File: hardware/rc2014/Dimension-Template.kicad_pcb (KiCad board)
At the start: 2 copper layers, 99.1 x 49.9 mm, 3 parts

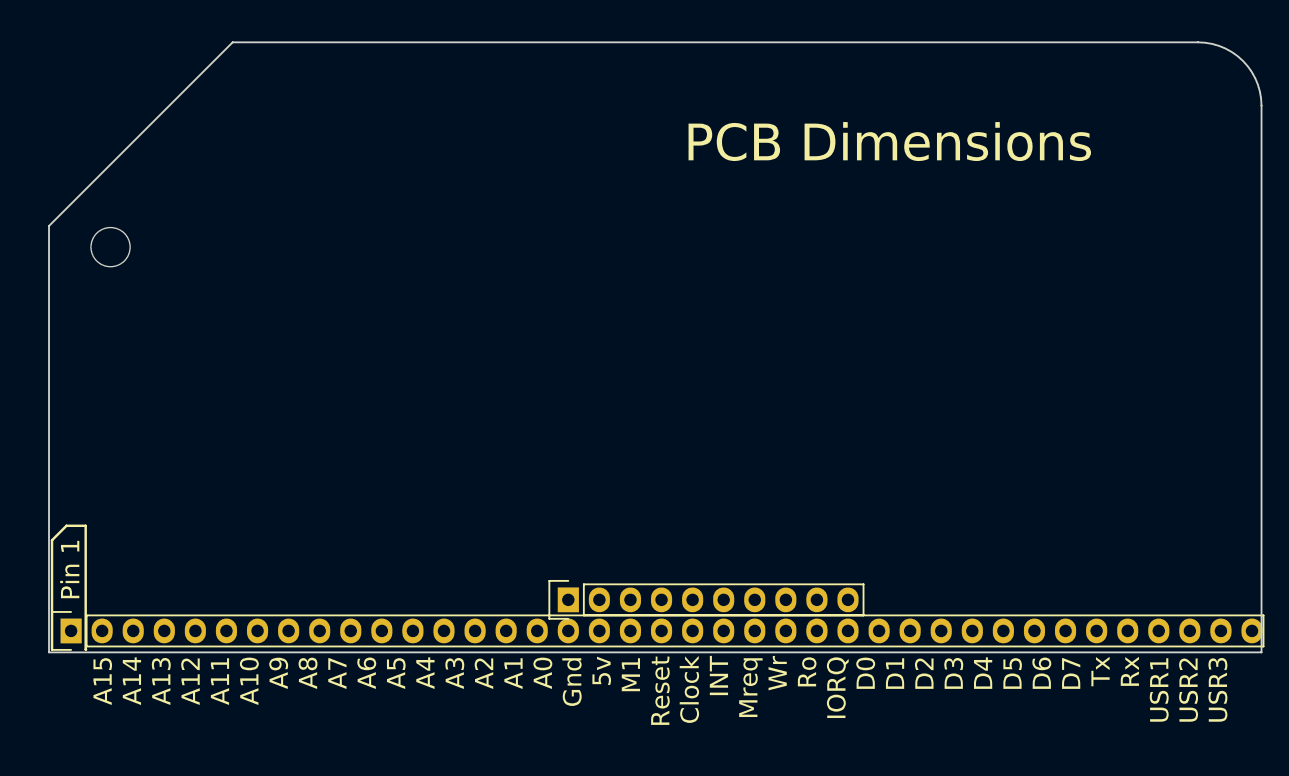
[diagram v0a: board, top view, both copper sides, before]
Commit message: more more cleaning
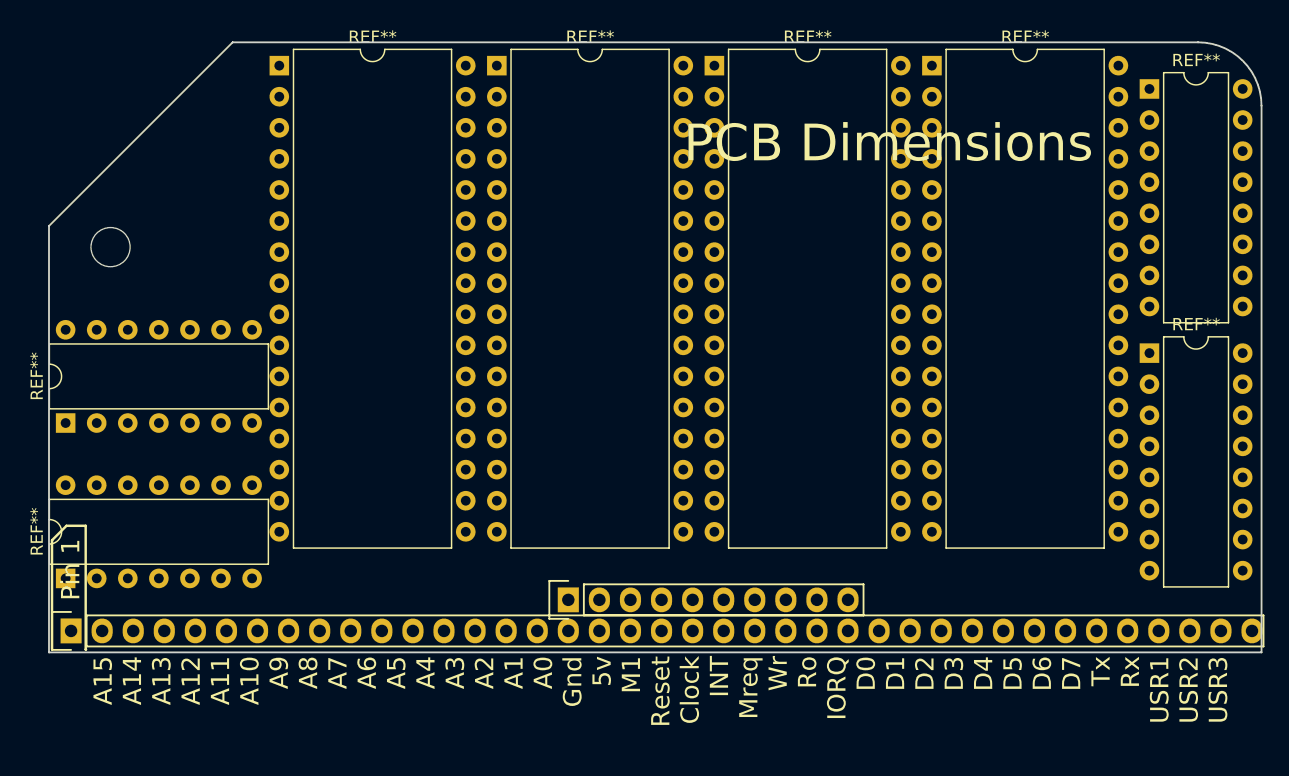
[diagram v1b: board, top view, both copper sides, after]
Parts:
- added REF**: DIP-14_W7.62mm, Package_DIP:DIP-14_W7.62mm, F.Cu at (155.3, 134.6)
- added REF**: DIP-14_W7.62mm, Package_DIP:DIP-14_W7.62mm, F.Cu at (155.3, 147.3)
- added REF**: DIP-16_W7.62mm, Package_DIP:DIP-16_W7.62mm, F.Cu at (243.8, 128.9)
- added REF**: DIP-16_W7.62mm, Package_DIP:DIP-16_W7.62mm, F.Cu at (243.8, 107.3)
- added REF**: DIP-32_W15.24mm, Package_DIP:DIP-32_W15.24mm, F.Cu at (226.1, 105.4)
- added REF**: DIP-32_W15.24mm, Package_DIP:DIP-32_W15.24mm, F.Cu at (208.3, 105.4)
- added REF**: DIP-32_W15.24mm, Package_DIP:DIP-32_W15.24mm, F.Cu at (190.5, 105.4)
- added REF**: DIP-32_W15.24mm, Package_DIP:DIP-32_W15.24mm, F.Cu at (172.7, 105.4)

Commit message: Working on 2-board 7220
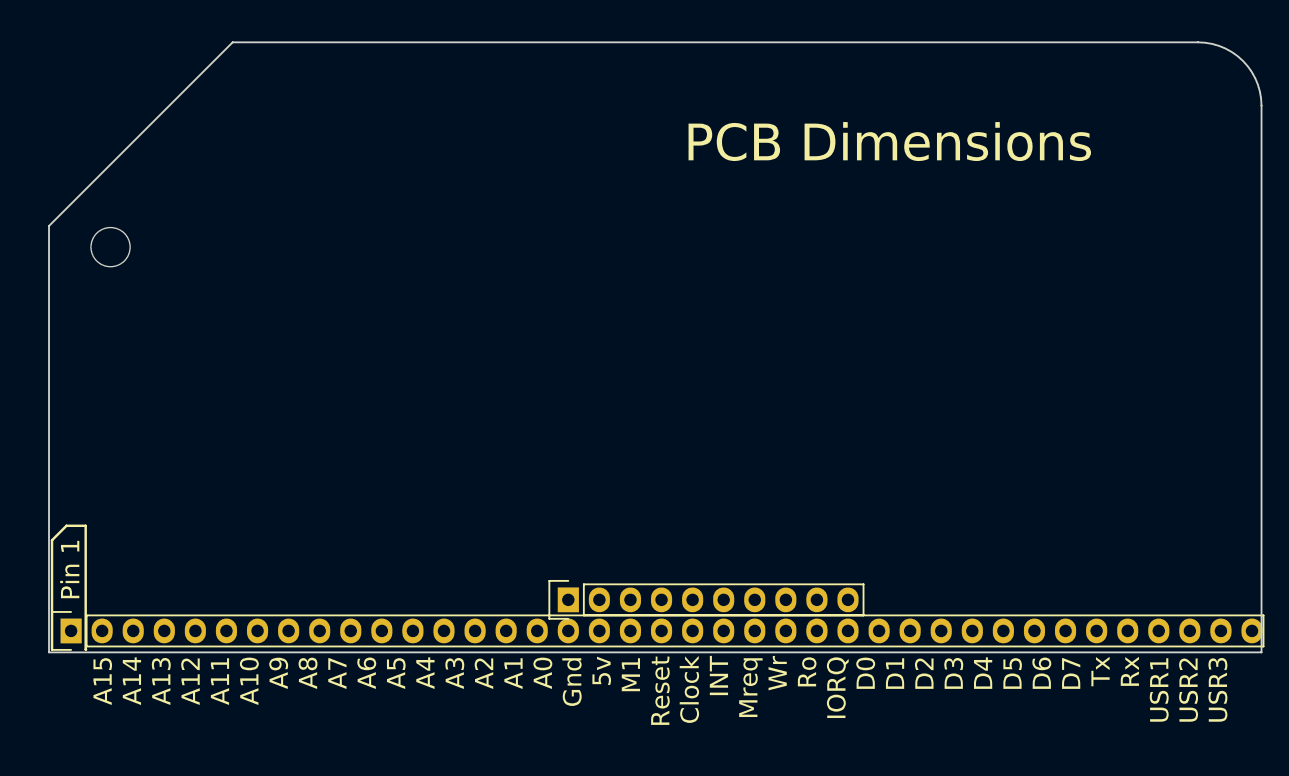
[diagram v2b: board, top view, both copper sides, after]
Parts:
- removed REF** (x2): DIP-14_W7.62mm, Package_DIP:DIP-14_W7.62mm
- removed REF** (x2): DIP-16_W7.62mm, Package_DIP:DIP-16_W7.62mm
- removed REF** (x4): DIP-32_W15.24mm, Package_DIP:DIP-32_W15.24mm
